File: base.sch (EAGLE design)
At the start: 20 parts

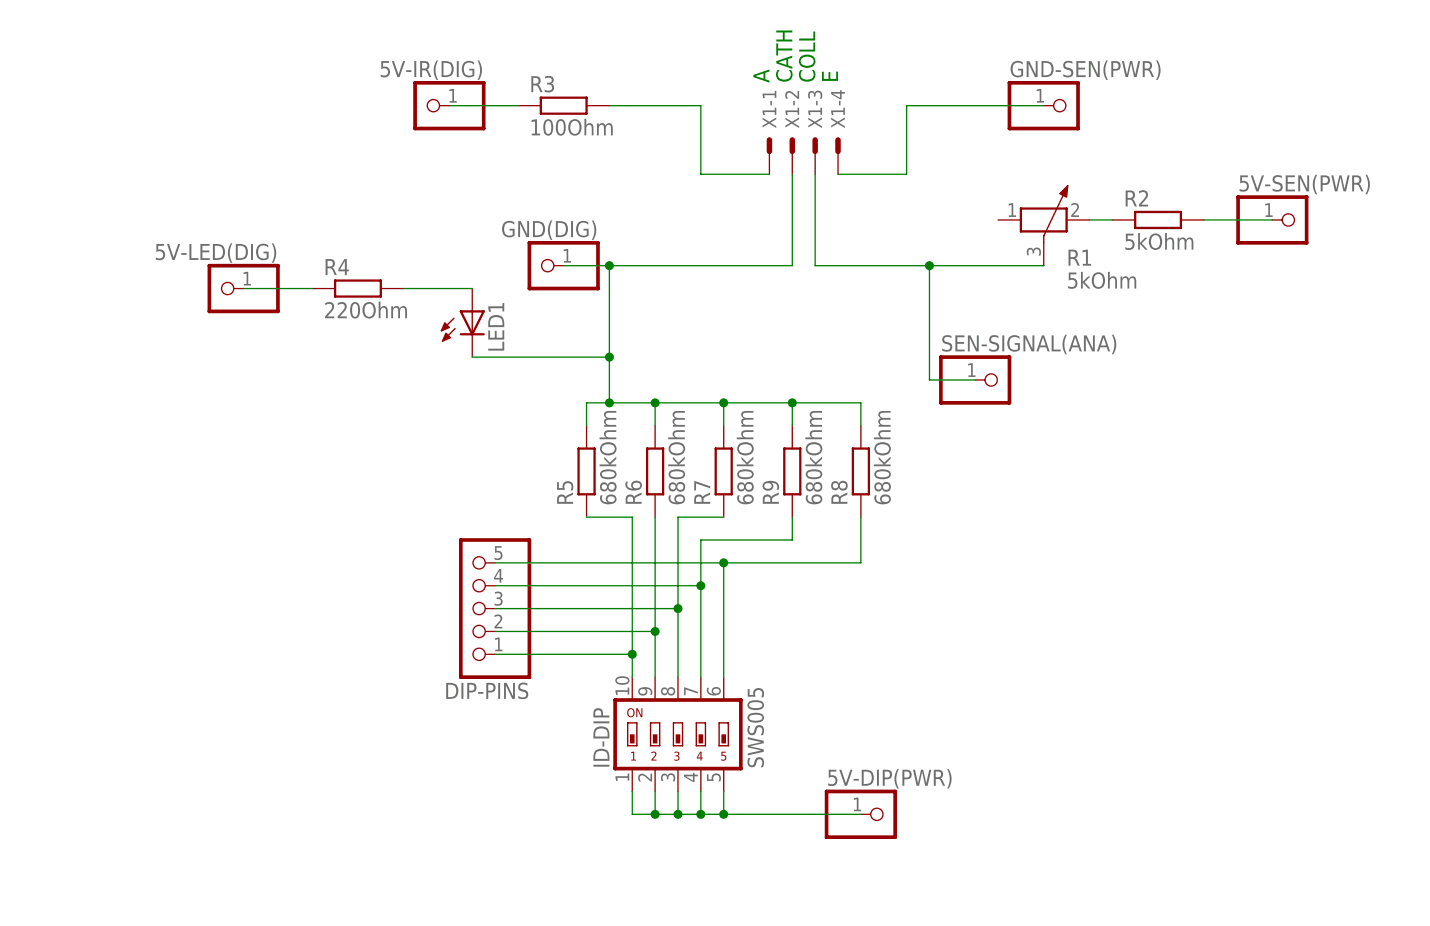
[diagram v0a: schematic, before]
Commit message: changed routing
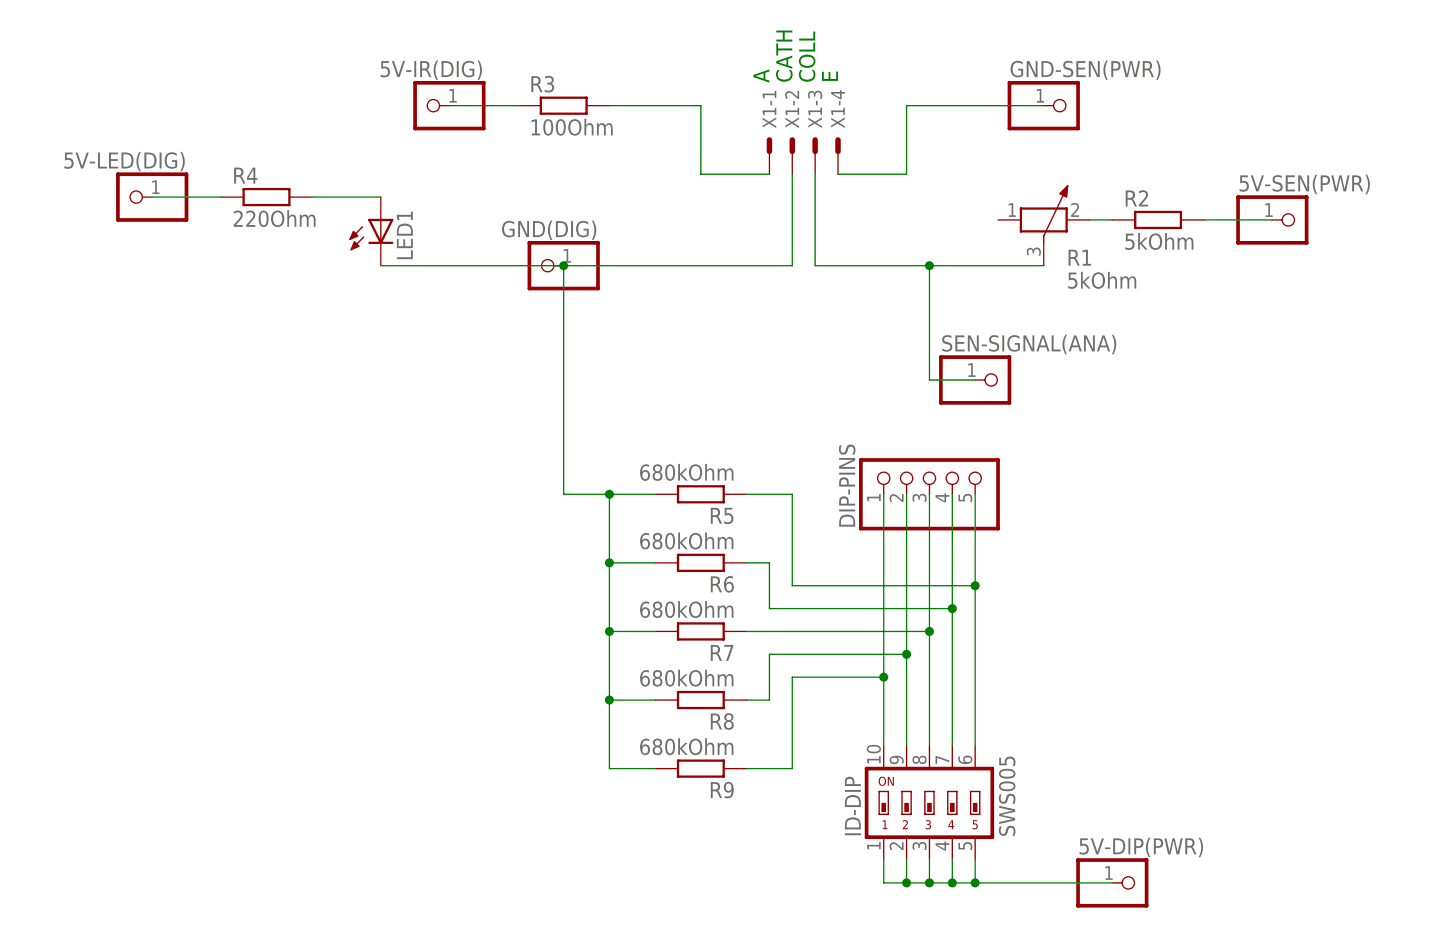
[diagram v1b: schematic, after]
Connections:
- removed net N$16 (its old number): DIP-PINS.5, ID-DIP.6, R8.1
- new net N$15: DIP-PINS.5, ID-DIP.6, R5.1
- net N$11: now also R9.1; no longer R5.1
- net N$12: now also R8.1; no longer R6.1
- net N$14: now also R6.1; no longer R9.1
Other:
- moved on the sheet: 5V-DIP(PWR), 5V-LED(DIG), DIP-PINS, ID-DIP, LED1, R4, R5, R6, R7, R8, R9
